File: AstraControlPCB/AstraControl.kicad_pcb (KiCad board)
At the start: 4 copper layers, 102 x 96 mm, 153 parts, among them CN1 4P JST VH, CN10 JST_ZH_6PIN_1A_250V, CN2 4P JST VH, CN3 4P JST VH, CN4 4P JST ZH, CN5 4P JST ZH, CN6 4P JST ZH, CN7 JST_VH_8PIN_10A_250V, CN8 4P JST ZH, CN9 4P JST ZH, SW1 TS_Basic_Small, SW2 TS_Basic_Small, U1 ESP32-S3-WROOM-1U-N8, U2 NCP361SNT1G, U3 ST1S12GR, U4 USBLC6-2SC6, U5 SN65HVD1782DR, U6 TXB0104PWR

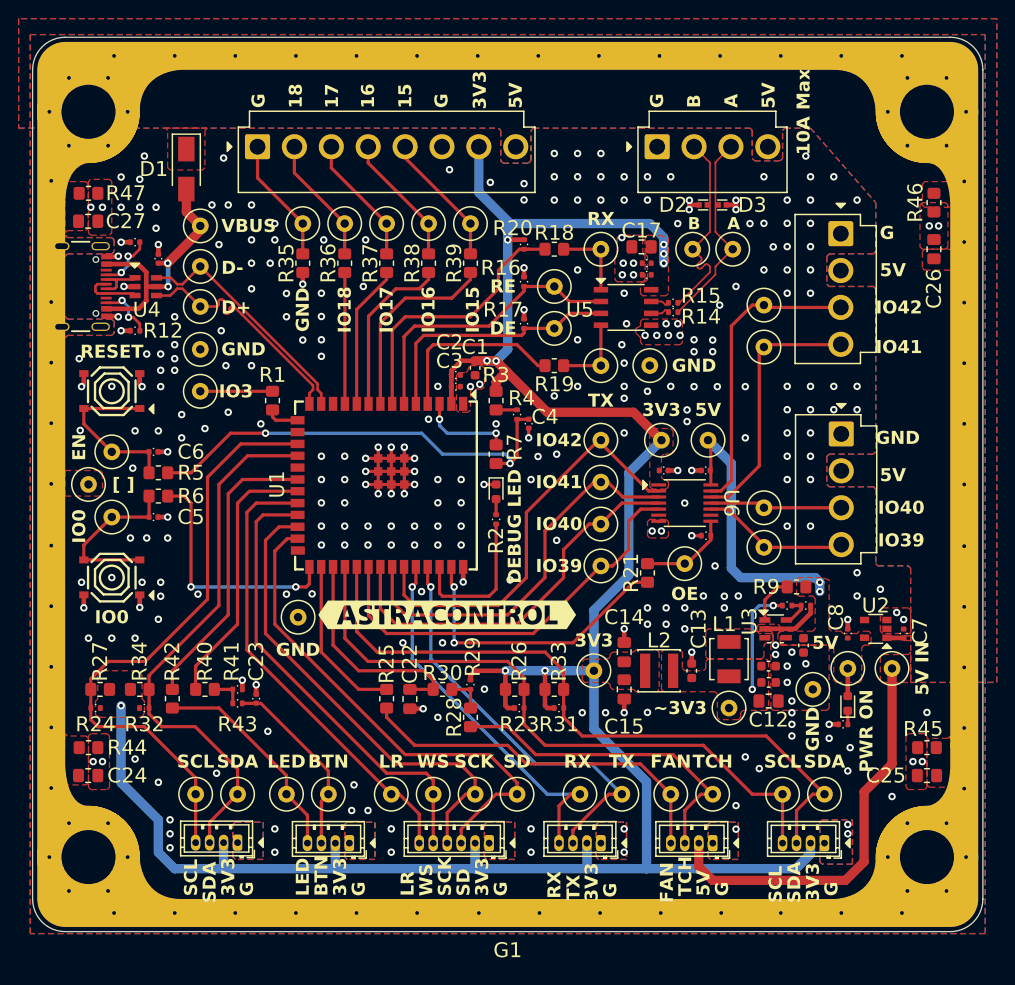
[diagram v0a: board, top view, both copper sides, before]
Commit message: Another redesign
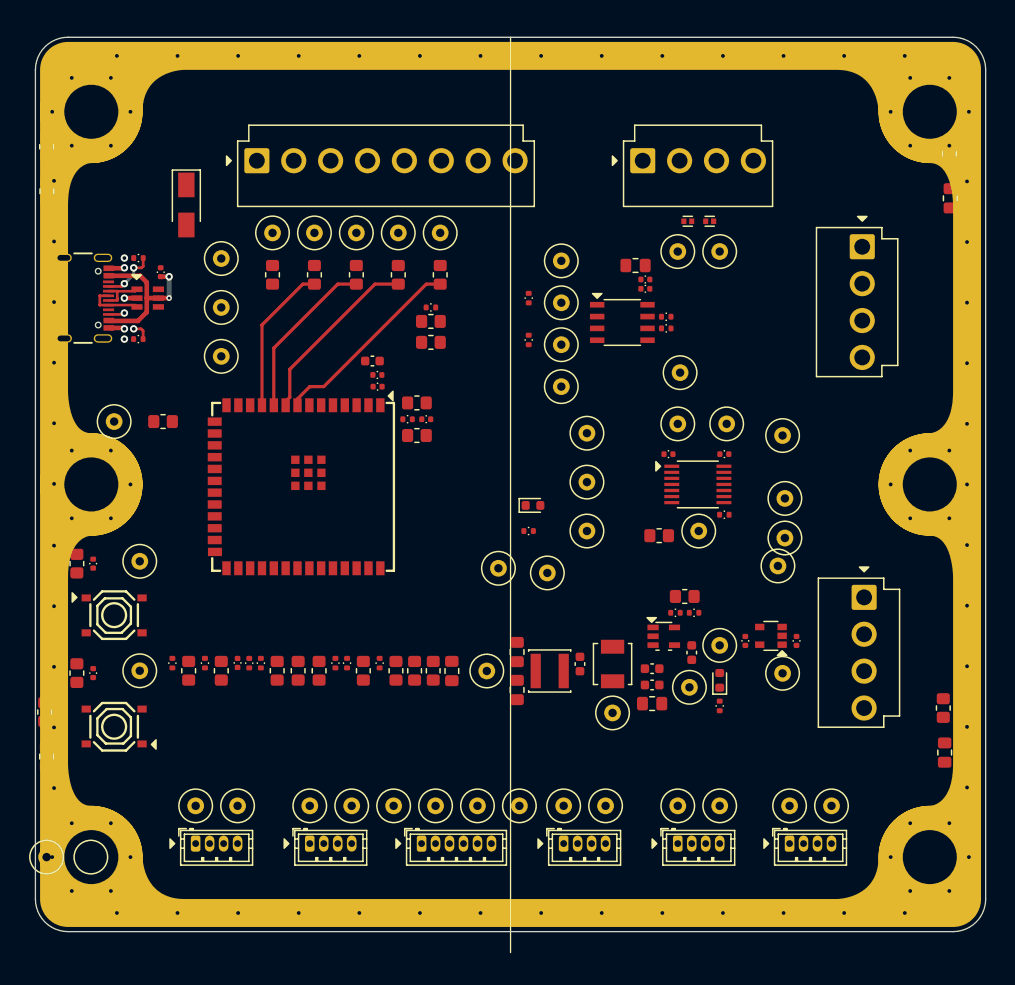
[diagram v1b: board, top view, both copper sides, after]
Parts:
- removed G1: ~, LiveAstra:AstraControl_Ground_Band
- removed kibuzzard-66D4B301: G***, kibuzzard-66D4B301
- added RING1: ~, LiveAstra:AstraControl_Ground_Ring, F.Cu at (149.8, 80.1)
- moved R44 64.7 mm to (100.0, 43.9), turned to 90 degrees
- moved R45 63.8 mm to (196.9, 44.6), turned to 90 degrees
- moved C24 62.9 mm to (100.0, 48.7), turned to 90 degrees
- moved C25 62.0 mm to (197.0, 49.4), turned to 90 degrees
- moved C27 57.6 mm to (100.0, 109.3), turned to 90 degrees
- moved R47 55.9 mm to (99.8, 104.6), turned to 90 degrees
- moved R46 54.3 mm to (196.3, 104.1)
- moved C26 54.0 mm to (196.4, 108.9), turned to 90 degrees
- moved TP11 40.3 mm to (100.0, 120.1)
- moved TP2 39.7 mm to (148.5, 89.1)
- moved TP10 34.0 mm to (104.8, 120.1)
- moved R33 25.3 mm to (129.3, 100.1), turned to 90 degrees
- moved R31 24.5 mm to (131.0, 99.3), turned to 90 degrees
- moved SW2 24.0 mm to (107.3, 94.2), turned to 0 degrees
- moved R6 20.9 mm to (103.3, 100.4), turned to -90 degrees
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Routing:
- net +3V3: track 256.7 -> 0.00 mm, vias 9 -> 0
- net /Block Diagram/Fan, Temperature and Screen/TEMP_I2C_SDA: track 74.5 -> 0.00 mm
- net GND: track 76.0 -> 4.59 mm, vias 308 -> 5
- net /Block Diagram/Fan, Temperature and Screen/TEMP_I2C_SCL: track 69.8 -> 0.00 mm
- net /Block Diagram/Fan, Temperature and Screen/SCREEN_I2C_SCL: track 65.5 -> 0.00 mm
- net /Block Diagram/Fan, Temperature and Screen/SCREEN_I2C_SDA: track 58.5 -> 0.00 mm
- net /Block Diagram/Button, Status LED, UART and I2S/I2S_SD: track 54.2 -> 0.00 mm
- net /Block Diagram/Button, Status LED, UART and I2S/I2S_SCK: track 51.7 -> 0.00 mm
- net /Block Diagram/Button, Status LED, UART and I2S/I2S_WS: track 49.7 -> 0.00 mm
- net /Block Diagram/Button, Status LED, UART and I2S/I2S_LR: track 49.5 -> 0.00 mm
- net /Block Diagram/MCU Enable and Boot/EN_DELAY: track 47.9 -> 0.00 mm, vias 2 -> 0
- net +5V_IN: track 45.5 -> 0.00 mm
- net /Block Diagram/Button, Status LED, UART and I2S/UART_TX: track 45.3 -> 0.00 mm, vias 1 -> 0
- net /Block Diagram/3V3 to 5V Logic Shifter/3V3_IO_1: track 44.7 -> 0.00 mm
- net /Block Diagram/3V3 to 5V Logic Shifter/3V3_IO_4: track 44.5 -> 0.00 mm
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- removed copper zone on F.Cu, net +3V3
- removed copper zone on F.Cu, net +5V
- removed copper zone on B.Cu, net +5V_IN
- removed copper zone on F.Cu, net +5V_IN
- removed copper zone on F.Cu, net /Block Diagram/5V to 3.3V/SW_OUT
- removed copper zone on F.Cu, net /Block Diagram/5V to 3.3V/SW_OUT_UNFILTERED
- removed copper zone on B.Cu, net CHASSIS
- removed copper zone on F.Cu, net CHASSIS
- removed copper zone on B.Cu, net GND
- removed copper zone on F.Cu, net GND
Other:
- board text removed: "10A Max"
- board text removed: "15"
- board text removed: "16"
- board text removed: "17"
- board text removed: "18"
- board text removed: "3V3"
- board text removed: "5V"
- board text removed: "5V IN"
- board text removed: "A"
- board text removed: "B"
- board text removed: "BTN"
- board text removed: "D+"
- board text removed: "D-"
- board text removed: "DE"
- board text removed: "DEBUG LED"
- board text removed: "EN"
- board text removed: "FAN"
- board text removed: "G"
- board text removed: "GND"
- board text removed: "IO0"
- board text removed: "IO15"
- board text removed: "IO16"
- board text removed: "IO17"
- board text removed: "IO18"
- board text removed: "IO3"
- board text removed: "IO39"
- board text removed: "IO40"
- board text removed: "IO41"
- board text removed: "IO42"
- board text removed: "JLCJLCJLCJLC"
- board text removed: "LED"
- board text removed: "LR"
- board text removed: "OE"
- board text removed: "PWR ON"
- board text removed: "RE"
- board text removed: "RESET"
- board text removed: "RX"
- board text removed: "SCK"
- board text removed: "SCL"
- board text removed: "SD"
- board text removed: "SDA"
- board text removed: "TCH"
- board text removed: "TX"
- board text removed: "VBUS"
- board text removed: "WS"
- board text removed: "[ ]"
- board text removed: "liveleds.io"
- board text removed: "~3V3"
